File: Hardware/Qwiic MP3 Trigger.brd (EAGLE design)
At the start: 25.4 x 50.8 mm, 108 parts, among them J14 MICRO-SD, J2 QWIIC_RIGHT_ANGLE, J3 PTH, J4 QWIIC_RIGHT_ANGLE, J7 ISP, J8 3.5mm Audio, J9 Poke-Home, U1 TPA2005D1, U3 AP2112-3.3V, U4 ATTINY84-ARDUINO, U5 MY1690X-16S

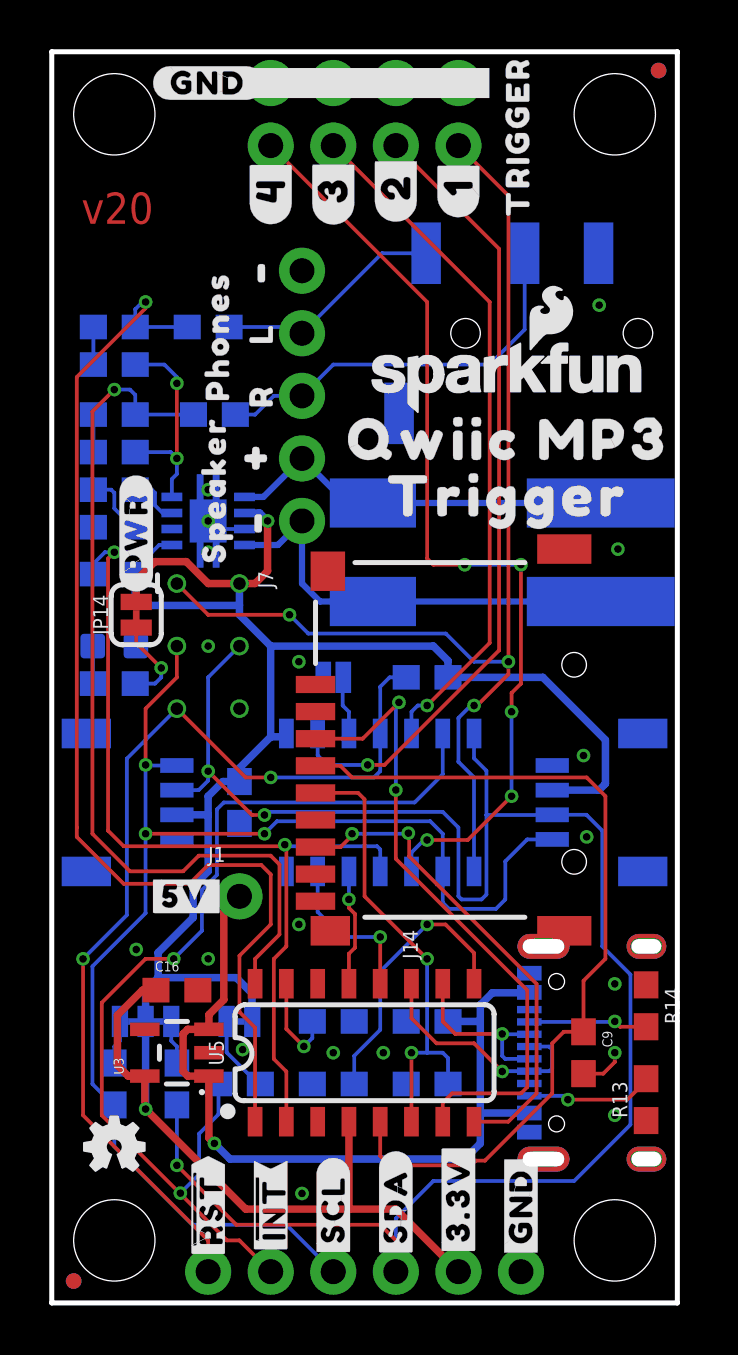
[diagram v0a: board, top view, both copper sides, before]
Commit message: Add v20 panel
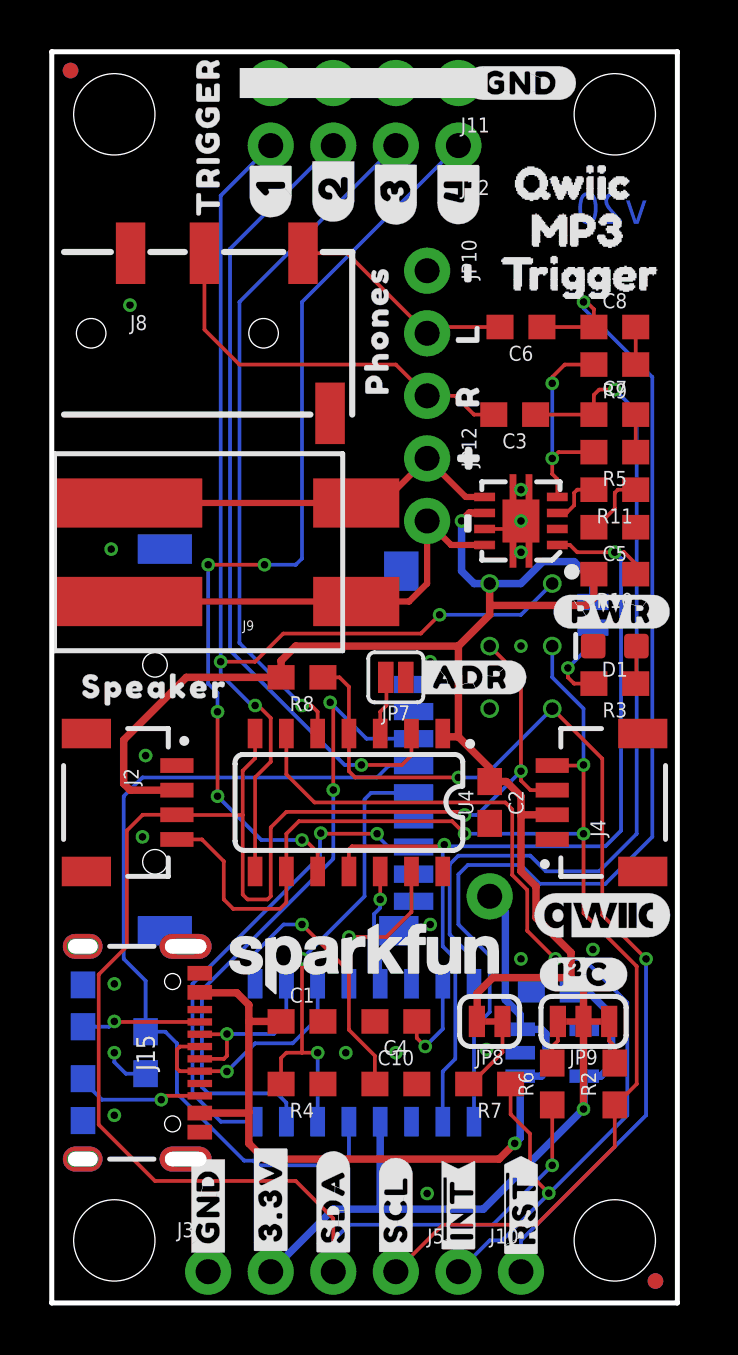
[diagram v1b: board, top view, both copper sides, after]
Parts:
- moved FRAME1 63.5 mm to (44.5, -34.3), flipped to the bottom
- moved J8 25.4 mm to (0.00, 39.4), flipped to the top
- moved JP1 23.9 mm to (0.76, 50.0), flipped to the bottom
- moved JP6 23.9 mm to (0.76, 50.0), flipped to the top
- moved JP2 23.6 mm to (24.5, 0.89), flipped to the top
- moved JP5 23.6 mm to (24.5, 0.89), flipped to the bottom
- moved R13 22.9 mm to (1.27, 8.26), flipped to the bottom
- moved R14 22.9 mm to (1.27, 12.1), flipped to the bottom
- moved C5 20.3 mm to (22.9, 31.5), flipped to the top
- moved C7 20.3 mm to (22.9, 36.1), flipped to the top
- moved C8 20.3 mm to (22.9, 39.6), flipped to the top
- moved D1 20.3 mm to (22.9, 26.7), flipped to the top
- moved JP11 20.3 mm to (2.54, 2.54), flipped to the top
- moved JP13 20.3 mm to (22.9, 2.54), flipped to the top
- moved JP3 20.3 mm to (2.54, 48.3), flipped to the top
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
